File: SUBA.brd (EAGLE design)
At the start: 85 x 70 mm, 19 parts, among them J3 PH_A_T, T1 2N2222

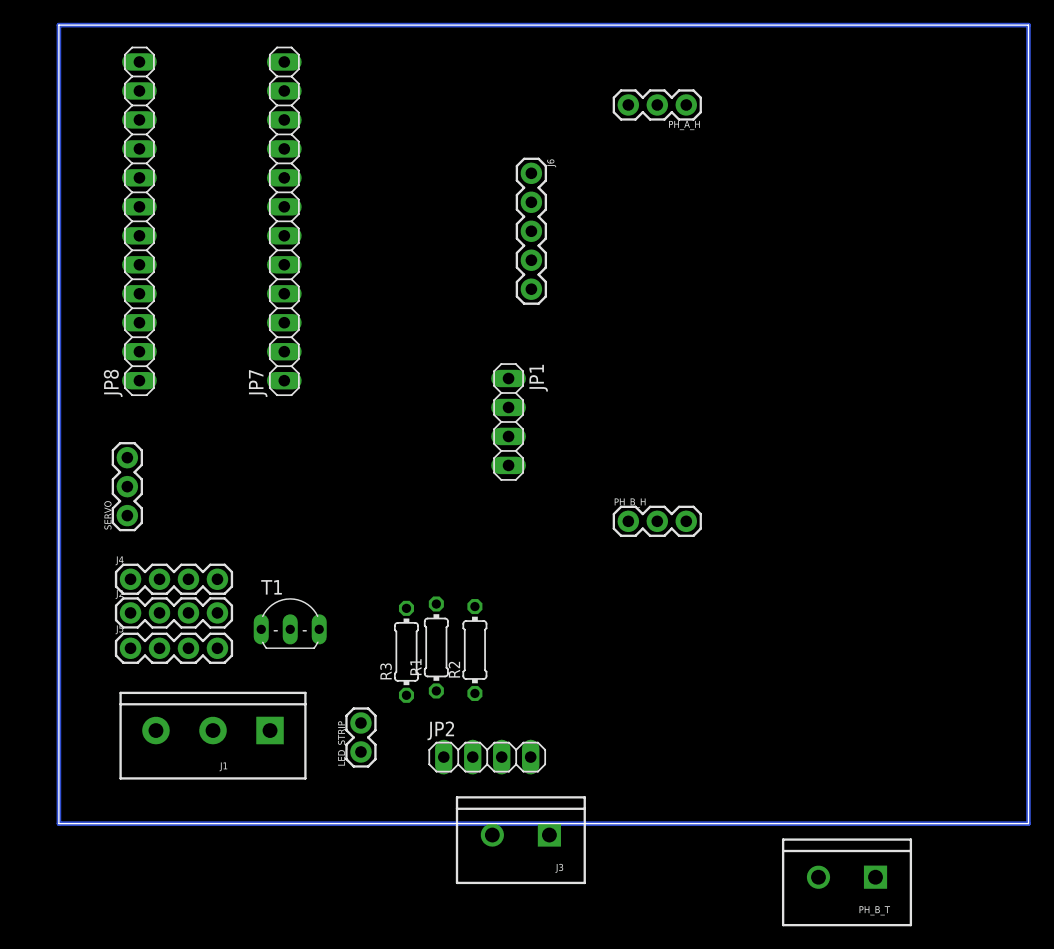
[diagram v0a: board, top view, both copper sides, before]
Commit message: SAFE
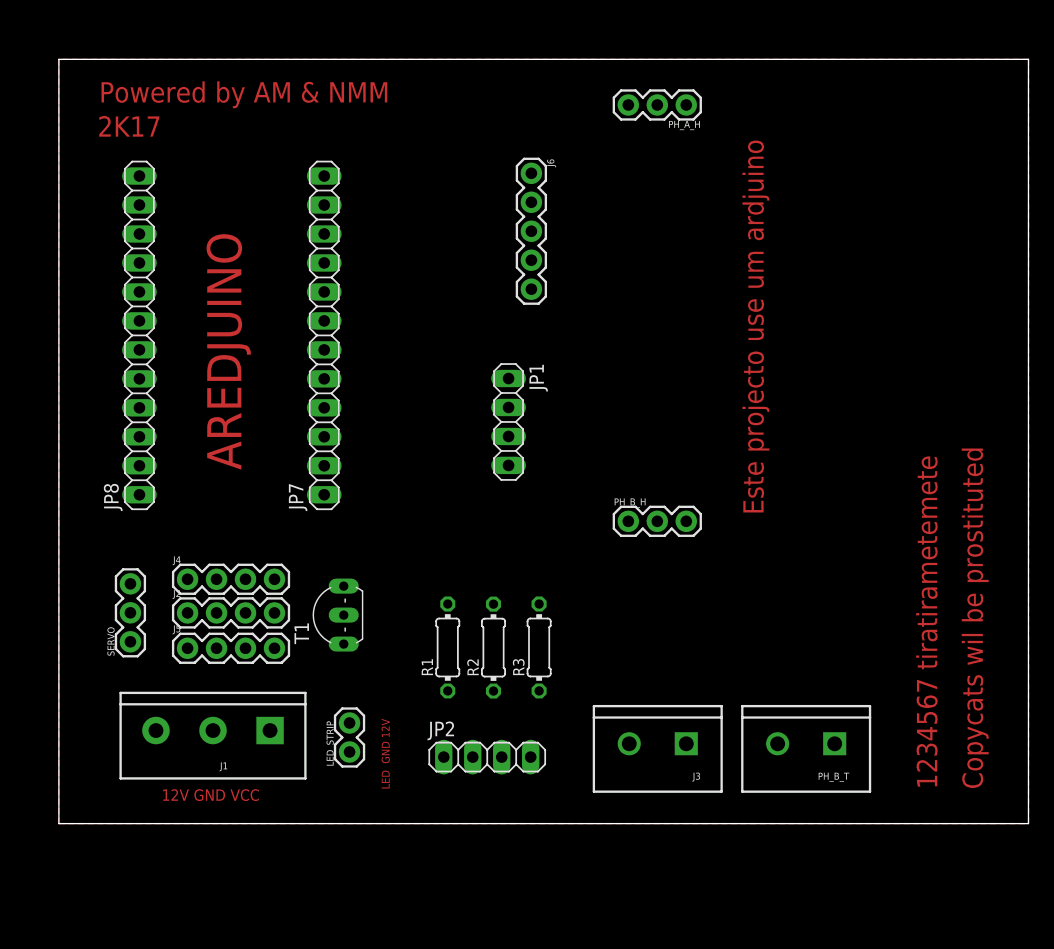
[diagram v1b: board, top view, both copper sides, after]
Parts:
- moved J3 14.4 mm to (55.0, 7.00)
- moved PH_B_T 12.2 mm to (68.0, 7.00)
- moved R3 11.6 mm to (42.1, 15.4)
- moved SERVO 11.1 mm to (6.27, 15.9)
- moved JP7 10.6 mm to (23.3, 42.8)
- moved JP8 10.0 mm to (7.06, 42.8)
- moved J2 5.00 mm to (11.3, 18.5)
- moved J4 5.00 mm to (11.3, 21.4)
- moved J5 5.00 mm to (11.3, 15.4)
- moved T1 3.42 mm to (23.7, 18.3), turned to 90 degrees
- moved R2 1.64 mm to (38.1, 15.4)
- moved LED_STRIP 1.00 mm to (25.5, 6.28)
- moved R1 1.00 mm to (34.1, 15.4)
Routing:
- net N$15: track 310.0 -> 0.00 mm
- added copper zone on layer 1, net N$15
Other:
- board size 85 x 70 mm -> 85 x 67 mm
- board text added: "1234567 tiratirametemete"
- board text added: "12V GND VCC"
- board text added: "2K17"
- board text added: "AREDJUINO"
- board text added: "Copycats wil be prostituted"
- board text added: "Este projecto use um ardjuino"
- board text added: "LED GND 12V"
- board text added: "Powered by AM & NMM"
